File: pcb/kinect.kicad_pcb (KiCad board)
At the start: 2 copper layers, 90 x 26 mm, 22 parts, among them J2 USB_C_Receptacle_USB2.0_16P, J3 Conn_02x05_Odd_Even, U1 LM3670MFX-1.8, U2 AP63203WU

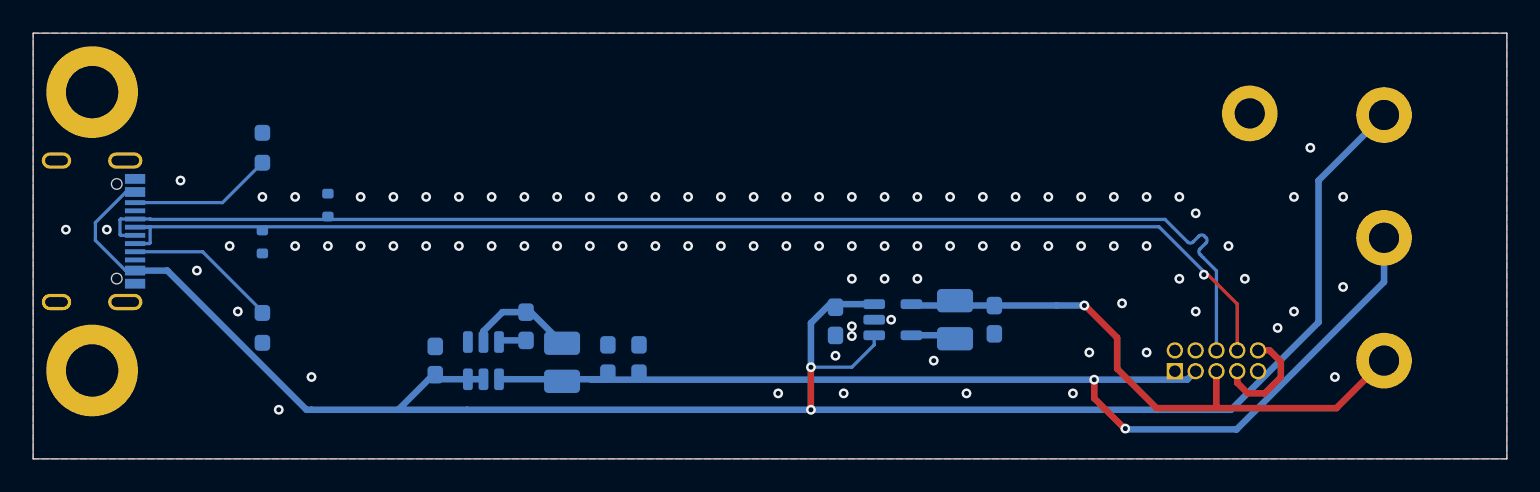
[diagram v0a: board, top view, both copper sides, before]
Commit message: Beautified the design.
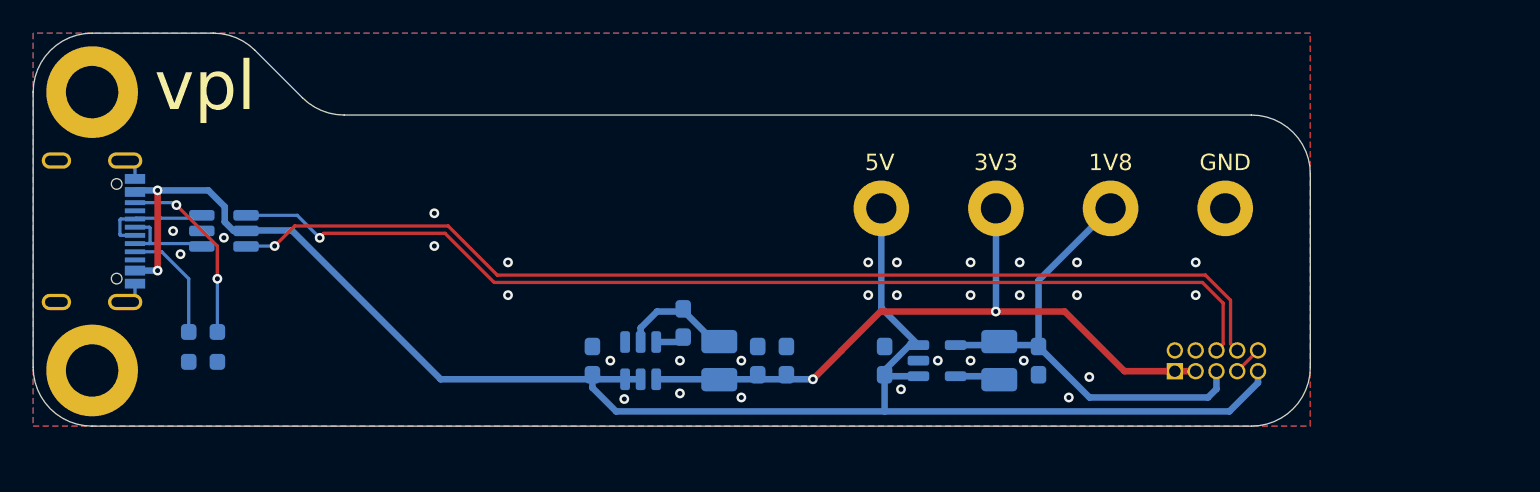
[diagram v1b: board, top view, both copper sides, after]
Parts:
- removed D1, D2: LESD5D5.0CT1G-ES, Diode_SMD:D_SOD-523
- added U3: USBLC6-2SC6, Package_TO_SOT_SMD:SOT-23-6_Handsoldering, B.Cu at (61.6, 62.1)
- C2: value 4u7 -> 10u
- J3: value Conn_02x05_Odd_Even -> Female Header 2x5P, P=1.27mm
- L1, L2: value 4u7 -> L 4u7
- moved TP3 31.2 mm to (101.8, 60.7)
- moved TP2 23.8 mm to (108.8, 60.7)
- moved TP1 19.1 mm to (115.8, 60.7)
- moved R2 12.5 mm to (61.2, 69.2), turned to -90 degrees
- moved C4 9.60 mm to (89.7, 67.7)
- moved L2 9.60 mm to (91.9, 70.0)
- moved C7 9.60 mm to (84.2, 70.0)
- moved U2 9.60 mm to (87.1, 70.0)
- moved C5 9.15 mm to (94.2, 70.0)
- moved C6 9.00 mm to (96.0, 70.0)
- moved TP4 5.99 mm to (122.8, 60.7)
- moved R1 4.65 mm to (59.5, 69.2)
- moved C2 3.84 mm to (102.0, 70.0), turned to 90 degrees
- moved C1 3.68 mm to (111.4, 70.0)
- moved L1 3.68 mm to (109.0, 70.0)
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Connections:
- J2 pad A6: /USB D+ -> Net-(J2-D+-PadA6)
- J2 pad A7: /USB D- -> Net-(J2-D--PadA7)
- J2 pad B6: /USB D+ -> Net-(J2-D+-PadA6)
- J2 pad B7: /USB D- -> Net-(J2-D--PadA7)
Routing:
- net +3V3: track 69.7 -> 42.5 mm
- net +5V: track 120.2 -> 103.6 mm
- net /USB D+: track 76.5 -> 65.2 mm, vias 0 -> 1
- net /USB D-: track 75.0 -> 65.8 mm
- net +1V8: track 36.0 -> 28.8 mm, vias 1 -> 0
- net Net-(J2-D+-PadA6): track 0.00 -> 7.02 mm
- net Net-(J2-D--PadA7): track 0.00 -> 6.28 mm
- net GND: track 6.67 -> 3.67 mm, vias 90 -> 31
- net Net-(J2-CC2): track 8.78 -> 11.4 mm, vias 0 -> 2
- net Net-(J2-CC1): track 9.37 -> 7.21 mm
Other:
- board size 90 x 26 mm -> 78 x 24 mm
- board text added: "1V8"
- board text added: "3V3"
- board text added: "5V"
- board text added: "GND"
- board text removed: "JLCJLCJLCJLC"
